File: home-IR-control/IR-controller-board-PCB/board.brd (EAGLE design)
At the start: 40 x 40 mm, 7 parts, among them J2 USB-TYPE-C-31-M-12, U1 CH340C

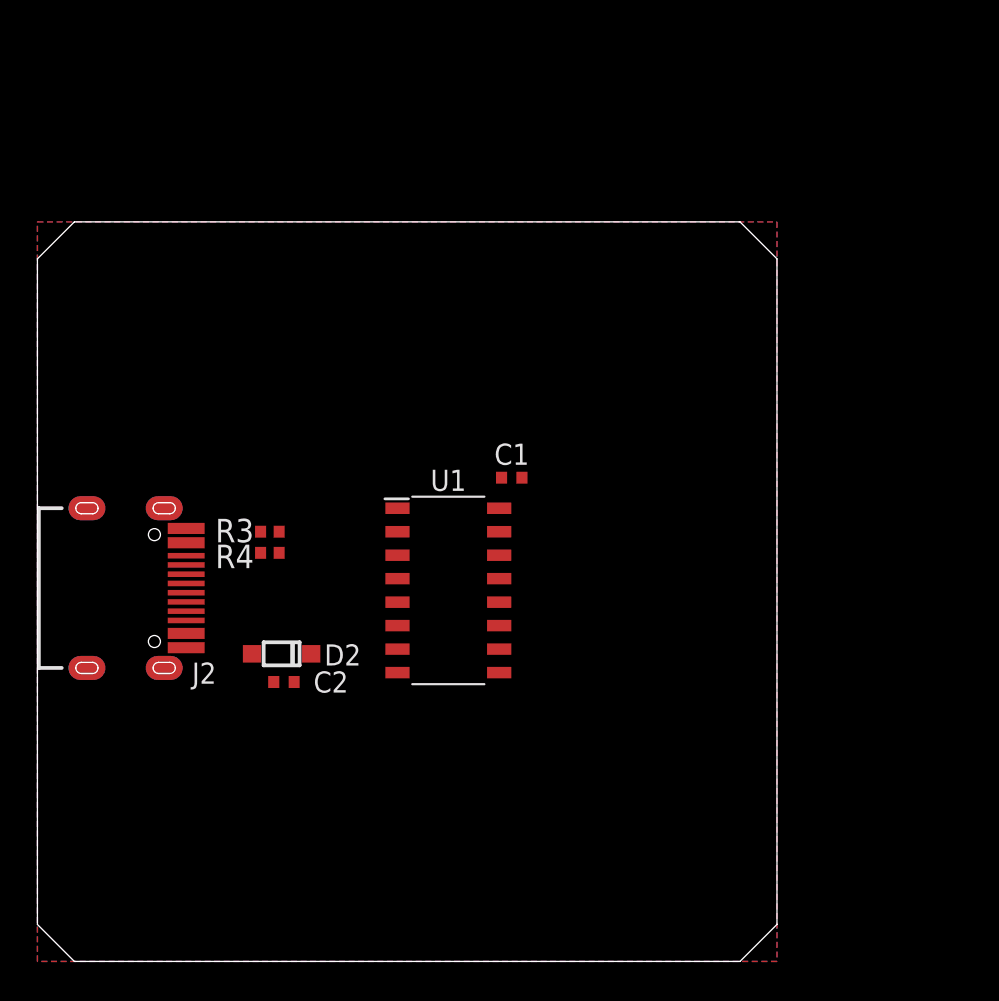
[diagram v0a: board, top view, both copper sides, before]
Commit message: PCB update
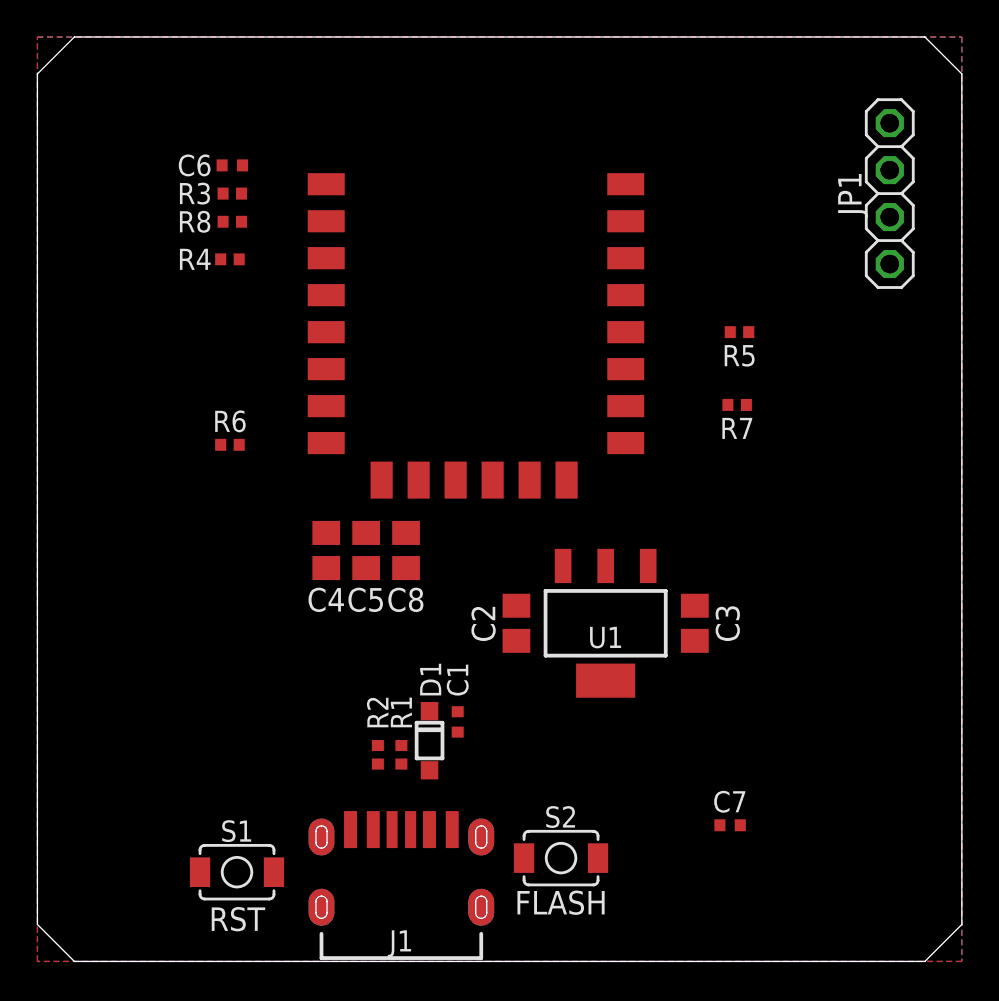
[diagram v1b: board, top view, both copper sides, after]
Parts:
- removed D2: B5819W, angrypig7-Diodes:SOD-123
- removed J2: USB-TYPE-C-31-M-12, angrypig7-Connectors:USB-TYPE-C-31-M-12
- added C3, C4, C5, C8: 22uF, angrypig7-RCL:C0805
- added C6, C7: 100nF, angrypig7-RCL:C0402
- added D1: B5819W, angrypig7-Diodes:SOD-123
- added J1: USB-TYPE-C-31-M-17, angrypig7-Connectors-USB:USB-TYPE-C-31-M-17
- added JP1: (no value), angrypig7-Connectors-PinHeads:1X04
- added M1: (no value), angrypig7-Boards:ESP8266-ESP12E
- added R1, R2: 4.7k, angrypig7-RCL:R0402
- added R5, R6, R7, R8: 10k, angrypig7-RCL:R0402
- added S1: RST, angrypig7-Switches:TACTILE_SWITCH_SMD_3.0X4.0MM
- added S2: FLASH, angrypig7-Switches:TACTILE_SWITCH_SMD_3.0X4.0MM
- C2: value 100nF -> 22uF; device angrypig7-RCL:C0402 -> angrypig7-RCL:C0805
- R3, R4: value 4.7k -> 10k
- U1: value CH340C -> AMS1117_SOT223; device angrypig7-IC:SOP-16_150MIL -> angrypig7-IC-Power:SOT-223
- moved R3 18.4 mm to (10.5, 41.5), turned to 0 degrees
- moved R4 16.0 mm to (10.4, 38.0), turned to 0 degrees
- moved C1 13.5 mm to (22.7, 13.0), turned to 270 degrees
- moved C2 13.0 mm to (25.9, 18.3), turned to 270 degrees
- moved U1 8.69 mm to (30.7, 18.3), turned to 90 degrees
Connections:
- removed net N$3: U1.14
- removed net N$4: U1.9
- removed net USB_N: J2.A7, J2.B7, U1.6
- removed net USB_P: J2.A6, J2.B6, U1.5
- new net ESP_ADC: M1.2, R8.2
- new net ESP_EN: M1.3, R4.2
- new net ESP_GPIO0: M1.12, R5.2, S2.1
- new net ESP_GPIO15: M1.10, R7.2
- new net ESP_GPIO2: M1.11, R6.2
- new net ESP_RST: C6.1, M1.1, R3.2, S1.1
- new net ESP_RST1: C7.1
- new net GND1: C7.2
- net 3V3: now also C3.1, C4.1, C5.1, C8.1, JP1.1, M1.8, R3.1, R4.1, R5.1, R6.1, U1.2; no longer C1.1, U1.16
- net 5V: now also C1.1, D1.C, U1.3; no longer D2.C
- net 5V_IN1: now also D1.A, J1.VBUS, J1.VBUS_2; no longer D2.A, J2.VBUS1, J2.VBUS2
- net GND: now also C3.2, C4.2, C5.2, C6.2, C8.2, J1.GND, J1.GND_2, J1.SHLD-B1, J1.SHLD-B2, J1.SHLD-B3, J1.SHLD-B4, J1.SHLD-T1, J1.SHLD-T2, J1.SHLD-T3, J1.SHLD-T4, JP1.4, M1.9, R1.1, R2.1, R7.1, R8.1, S1.2, S2.2; no longer J2.GND1, J2.GND2, J2.SHLD-B1, J2.SHLD-B2, J2.SHLD-B3, J2.SHLD-B4, J2.SHLD-T1, J2.SHLD-T2, J2.SHLD-T3, J2.SHLD-T4, R3.1, R4.1
- net N$1: now also J1.CC1, R2.2; no longer J2.A5, R3.2
- net N$2: now also J1.CC2, R1.2; no longer J2.B5, R4.2
- net UART_RX: now also JP1.2, M1.15; no longer U1.3
- net UART_TX: now also JP1.3, M1.16; no longer U1.2
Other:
- board size 40 x 40 mm -> 50 x 50 mm
- board text added: "FLASH"
- board text added: "RST"
